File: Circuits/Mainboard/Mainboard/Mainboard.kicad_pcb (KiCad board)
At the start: 2 copper layers, 170 x 170 mm, 66 parts, among them IC1 LM74500QDDFRQ1, IC2 LM74500QDDFRQ1, IC3 2536030320001, IC6 TPS563300DRLR, IC7 TPS563300DRLR, J1 XT60PW-M, J10 B5P-VH_LF__SN_, J11 B6B-PH-K-S, J12 B5P-VH_LF__SN_, J13 B6B-PH-K-S, J14 B5P-VH_LF__SN_, J16 B5P-VH_LF__SN_, J17 Conn_01x04_Pin, J2 XT60PW-M, J23 Conn_01x04_Pin, J24 Conn_01x06_Pin, J25 Conn_01x06_Pin, J26 Conn_01x04_Pin, J27 Conn_01x04_Pin, J3 Conn_01x06_Pin, J5 B6B-PH-K-S, J6 B5P-VH_LF__SN_, J7 B6B-PH-K-S, J8 Conn_01x06_Pin, J9 Conn_01x04_Pin, P1 66200621122, Q1 PSMN6R7-40MLDX, Q2 PSMN6R7-40MLDX, U1 NUCLEOH723ZG, U2 ADP121-AUJZ28R7

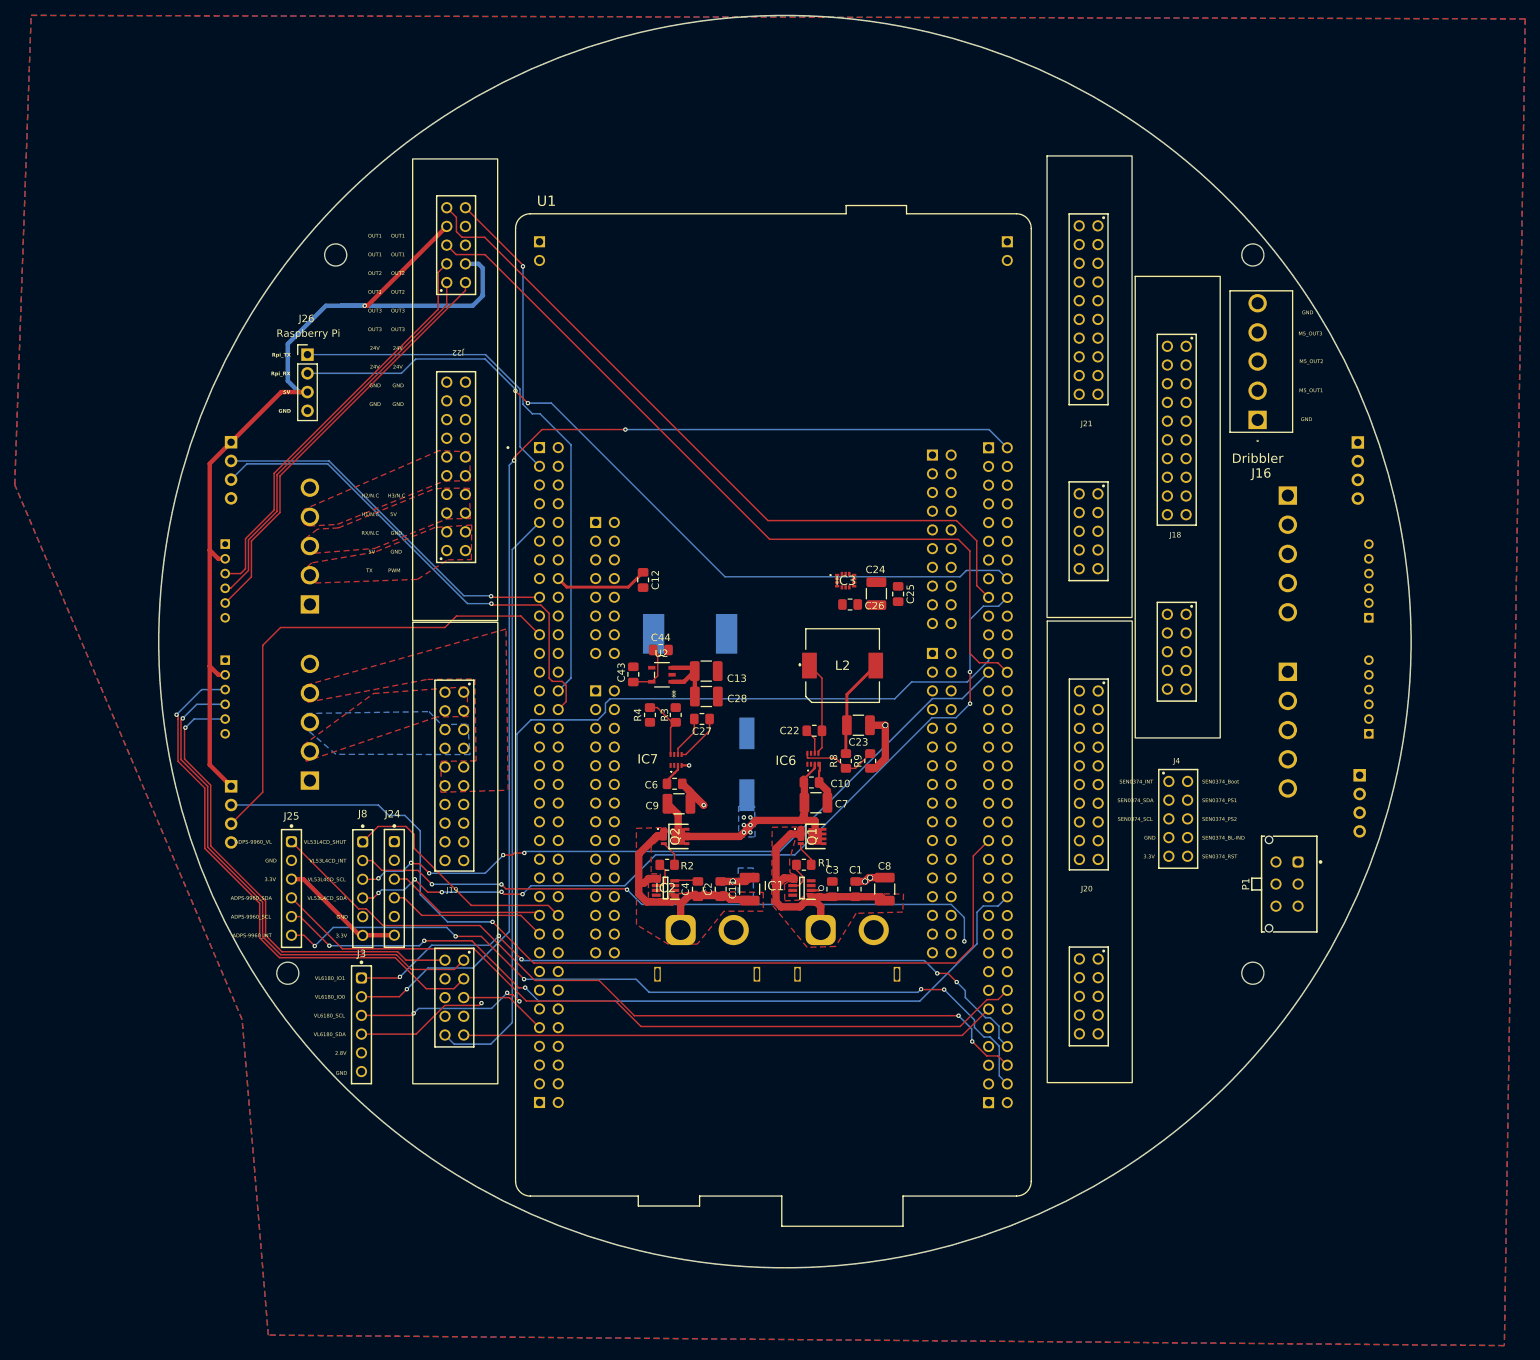
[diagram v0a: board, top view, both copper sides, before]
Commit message: Mainborad routing
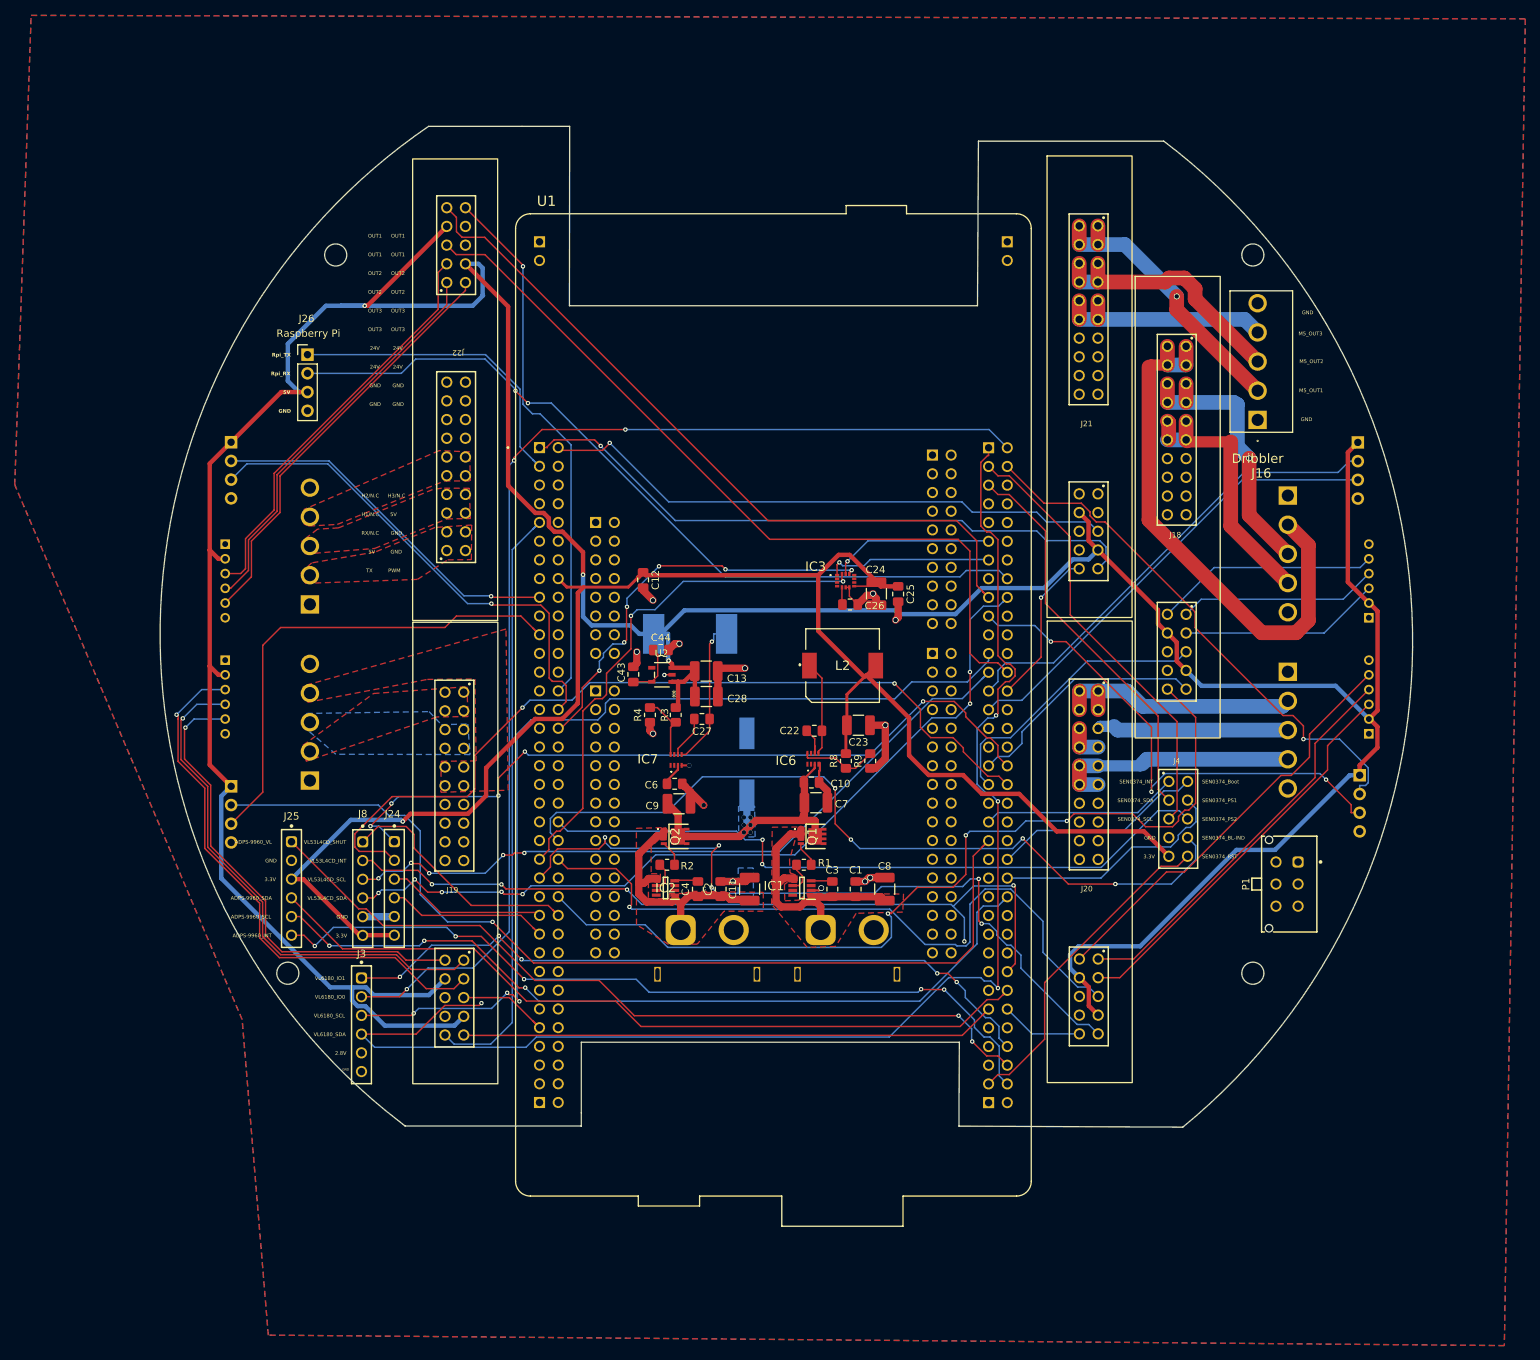
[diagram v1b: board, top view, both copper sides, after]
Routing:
- net 5V: track 140.9 -> 515.6 mm, vias 1 -> 3
- net 3.3V: track 43.6 -> 223.5 mm, vias 0 -> 1
- net /VL6180_SDA: track 18.0 -> 190.4 mm, vias 1 -> 4
- net /M2_PWM: track 0.00 -> 122.1 mm, vias 0 -> 3
- net /VL53L4CD2_INT: track 0.00 -> 115.1 mm, vias 0 -> 2
- net /SEN0374_BL-IND: track 0.00 -> 108.2 mm, vias 0 -> 4
- net /VL53L4CD2_SHUT: track 0.00 -> 104.3 mm, vias 0 -> 5
- net /M4_TX: track 0.00 -> 102.2 mm, vias 0 -> 5
- net /M4_RX: track 0.00 -> 95.1 mm, vias 0 -> 1
- net /SEN0374_PS2: track 0.00 -> 93.7 mm, vias 0 -> 2
- net /M5_TX: track 0.00 -> 86.8 mm, vias 0 -> 1
- net /M5_RX: track 0.00 -> 78.8 mm, vias 0 -> 1
- net /M2_OUT1: track 0.00 -> 73.8 mm
- net /M4_Encoder_A: track 0.00 -> 73.0 mm, vias 0 -> 1
- net WSENS_SDA: track 0.00 -> 70.9 mm, vias 0 -> 2
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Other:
- board size 170 x 170 mm -> 170 x 135.9 mm
